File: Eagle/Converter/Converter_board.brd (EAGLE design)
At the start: 100 x 80 mm, 12 parts

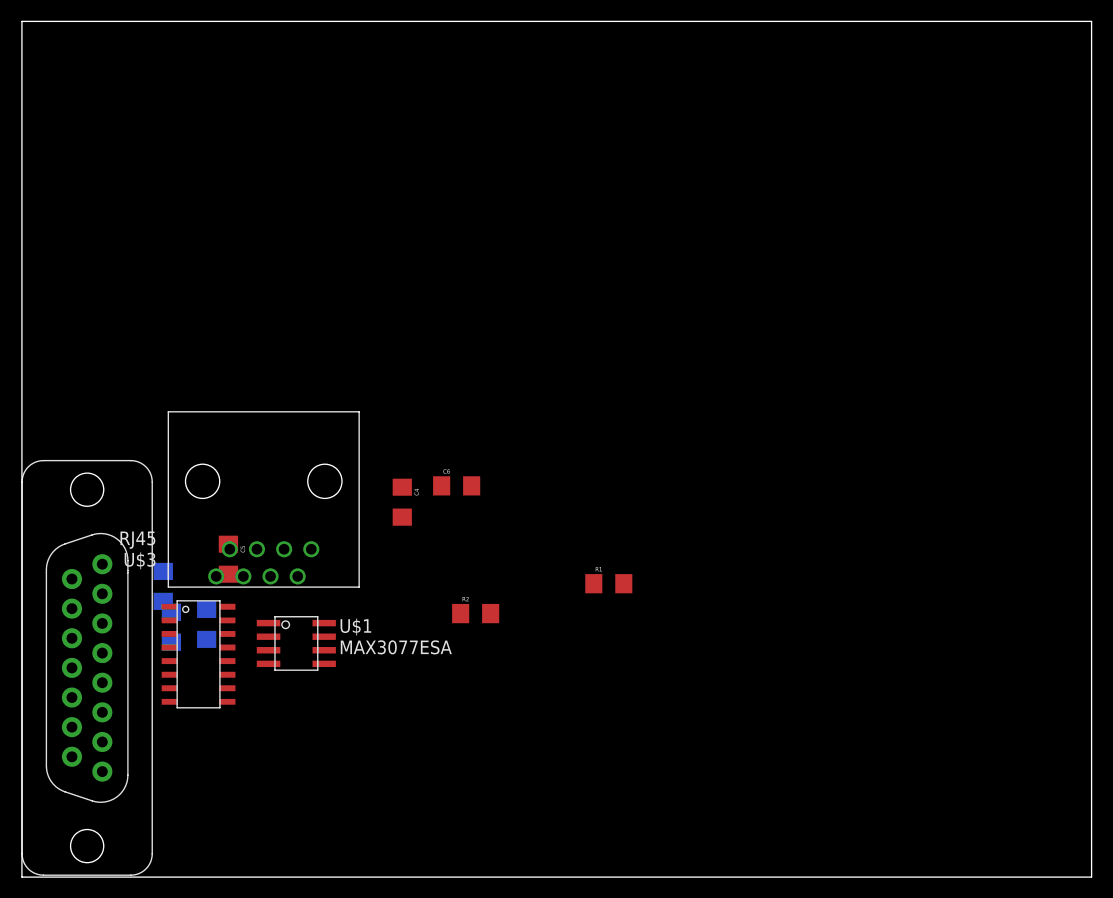
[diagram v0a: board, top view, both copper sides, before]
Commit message: routed board
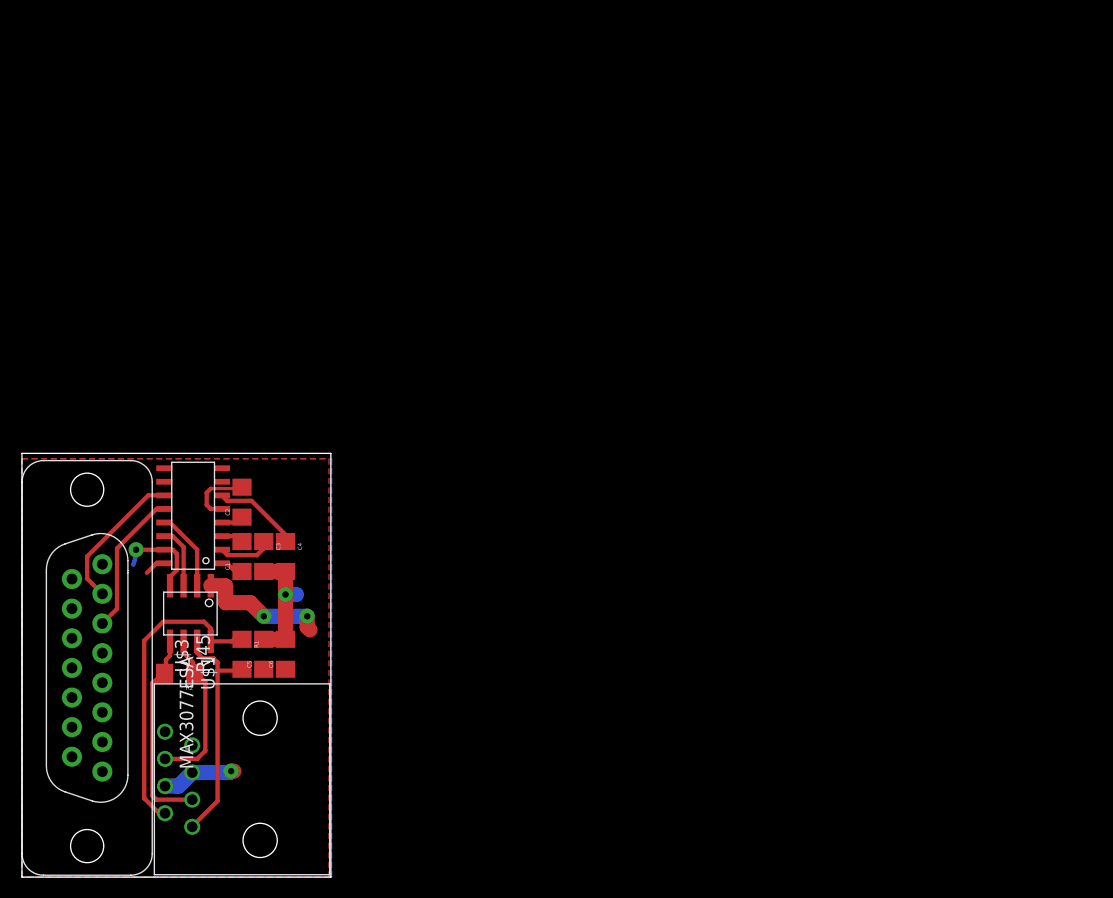
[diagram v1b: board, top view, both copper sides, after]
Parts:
- moved R1 34.9 mm to (20.6, 20.8), turned to 270 degrees
- moved R2 28.2 mm to (14.7, 19.1), turned to 180 degrees
- moved U$3 26.2 mm to (20.6, 9.14), turned to 90 degrees
- moved C6 22.5 mm to (24.6, 20.8), turned to 90 degrees
- moved C2 13.4 mm to (20.6, 35.1), flipped to the top, turned to 90 degrees
- moved U$2 13.0 mm to (16.0, 33.8), turned to 180 degrees
- moved C4 12.0 mm to (24.6, 30.0)
- moved U$1 10.3 mm to (15.7, 24.6), turned to 270 degrees
- moved C5 9.48 mm to (22.6, 20.8), turned to 90 degrees
- moved C3 8.29 mm to (22.6, 30.0), flipped to the top, turned to 270 degrees
- moved C1 7.88 mm to (20.6, 30.0), flipped to the top, turned to 90 degrees
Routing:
- net TRANS-: track 0.00 -> 28.7 mm
- net TRANS+: track 0.00 -> 22.0 mm
- net VCC: track 0.00 -> 21.5 mm, vias 0 -> 3
- net GND: track 0.00 -> 20.1 mm, vias 0 -> 2
- net REC+: track 0.00 -> 19.1 mm
- net REC-: track 0.00 -> 15.1 mm
- net T_IN1: track 0.00 -> 13.7 mm
- net R_OUT1: track 0.00 -> 13.5 mm
- net N$5: track 0.00 -> 8.32 mm
- net R_IN1: track 0.00 -> 7.50 mm
- net N$4: track 0.00 -> 6.24 mm
- net T_OUT1: track 0.00 -> 5.85 mm
- net N$6: track 0.00 -> 5.24 mm
- net N$2: track 0.00 -> 2.19 mm
- net N$3: track 0.00 -> 2.08 mm
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- added copper zone on layer 16, net GND
- added copper zone on layer 1, net VCC
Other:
- board size 100 x 80 mm -> 28.9 x 39.6 mm
